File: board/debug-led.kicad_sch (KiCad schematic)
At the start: 21 parts, among them U22 74HC373, U23 74HC373, U24 DA56-11SRWA

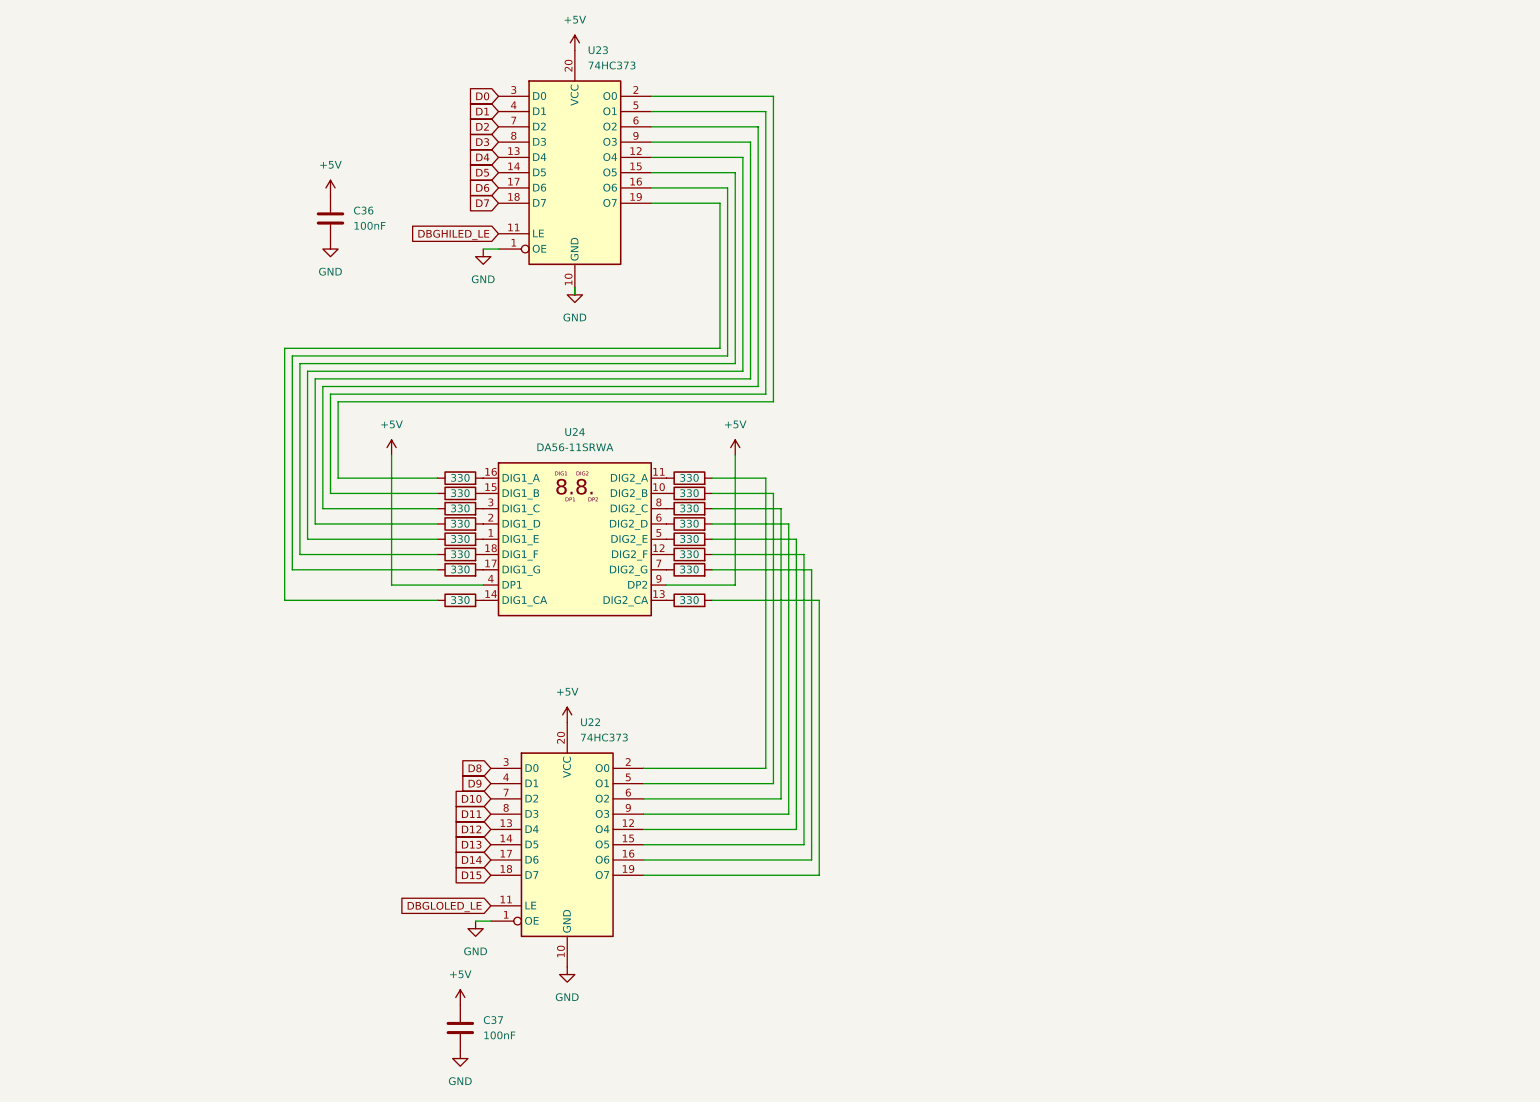
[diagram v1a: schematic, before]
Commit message: checkpoint
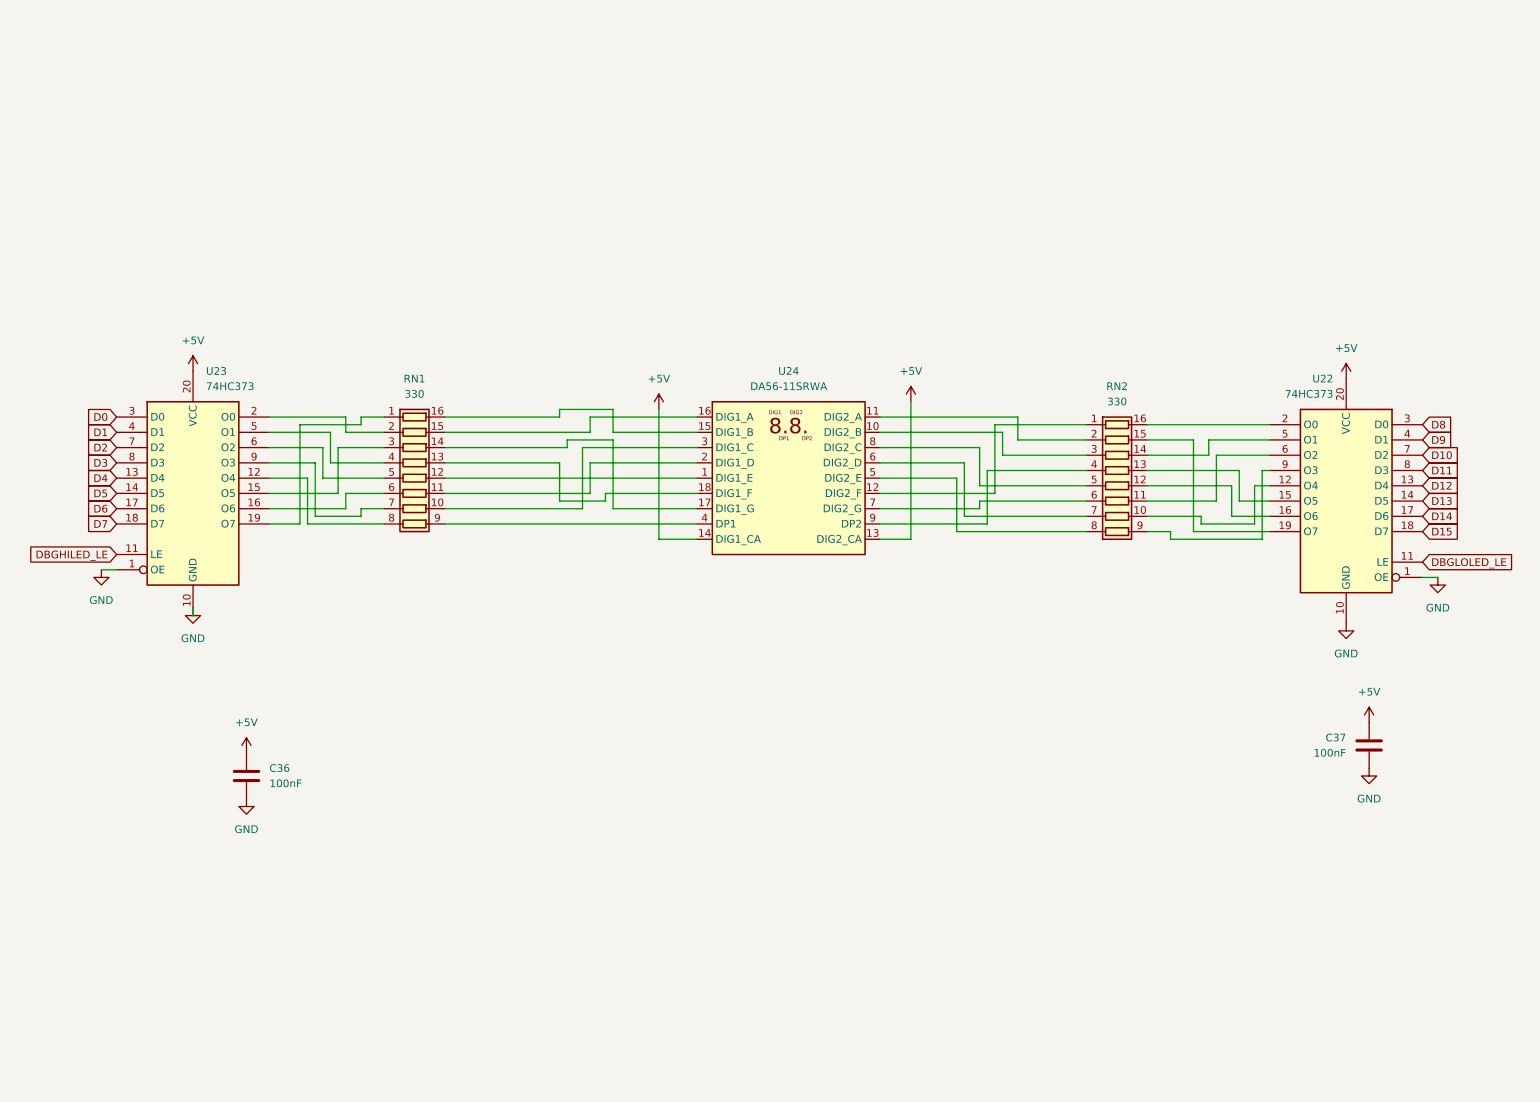
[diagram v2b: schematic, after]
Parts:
- removed R17, R18, R19, R20, R21, R22, R23, R24, R25, R26, R27, R28, R29, R30, R31, R32: 330, Resistor_THT:R_Axial_DIN0207_L6.3mm_D2.5mm_P10.16mm_Horizontal, symbol Device:R
- added RN1, RN2: 330, Package_DIP:DIP-16_W7.62mm, symbol Device:R_Pack08
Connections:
- net +5V: now also U24.13 (DIG2_CA), U24.14 (DIG1_CA); no longer U24.4 (DP1), U24.9 (DP2)
- net at U23.2 (O0): now also RN1.2 (R2.1)
- net at U24.16 (DIG1_A): now also RN1.15 (R2.2)
- net at U24.11 (DIG2_A): now also RN2.2 (R2.1)
- net at U22.2 (O0): now also RN2.16 (R1.2)
- net at U22.12 (O4): now also RN2.10 (R7.2)
- net at U22.15 (O5): now also RN2.13 (R4.2)
- net at U22.16 (O6): now also RN2.12 (R5.2)
- net at U22.19 (O7): now also RN2.15 (R2.2)
- net at U22.5 (O1): now also RN2.14 (R3.2)
- net at U22.6 (O2): now also RN2.11 (R6.2)
- net at U22.9 (O3): now also RN2.9 (R8.2)
- net at U23.15 (O5): now also RN1.3 (R3.1)
- net at U24.18 (DIG1_F): now also RN1.13 (R4.2)
- net at U24.5 (DIG2_E): now also RN2.8 (R8.1)
- net at U24.7 (DIG2_G): now also RN2.6 (R6.1)
- net at U23.12 (O4): now also RN1.8 (R8.1)
- net at U23.16 (O6): now also RN1.6 (R6.1)
- net at U23.19 (O7): now also RN1.1 (R1.1)
- net at U23.5 (O1): now also RN1.4 (R4.1)
- net at U23.6 (O2): now also RN1.5 (R5.1)
- net at U23.9 (O3): now also RN1.7 (R7.1)
- net at U24.17 (DIG1_G): now also RN1.14 (R3.2)
- net at U24.2 (DIG1_D): now also RN1.11 (R6.2)
- net at U24.15 (DIG1_B): now also RN1.16 (R1.2)
- net at U24.8 (DIG2_C): now also RN2.5 (R5.1)
- net at U24.3 (DIG1_C): now also RN1.10 (R7.2)
- net at U24.6 (DIG2_D): now also RN2.7 (R7.1)
- net at U24.1 (DIG1_E): now also RN1.12 (R5.2)
- net at U24.10 (DIG2_B): now also RN2.3 (R3.1)
- net at U24.12 (DIG2_F): now also RN2.1 (R1.1)
- new net: RN1.9 (R8.2), U24.4 (DP1)
- new net: RN2.4 (R4.1), U24.9 (DP2)
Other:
- moved on the sheet: C36, C37, U22, U23, U24

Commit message: checkpoint
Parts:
- RN1, RN2: digikey (none) -> https://www.digikey.com/en/products/detail/bourns-inc/4116R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
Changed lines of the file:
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@@
+			)
+		)
+		(property "digikey" "https://www.digikey.com/en/products/detail/bourns-inc/4116R-R2R-103LF/2565166"
+			(at 82.55 91.44 90)
+			(effects
+				(font
+					(size 1.27 1.27)
+				)
+				(hide yes)
 			)
 		)
@@
 			(effects
 				(font
+					(size 1.27 1.27)
+				)
+				(hide yes)
+			)
+		)
+		(property "digikey" "https://www.digikey.com/en/products/detail/bourns-inc/4116R-R2R-103LF/2565166"
+			(at 199.39 92.71 90)
+			(effects
+				(font
